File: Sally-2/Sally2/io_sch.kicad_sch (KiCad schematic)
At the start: 41 parts, among them J12 Drive 1-4, J13 OPT, J14 Special_Func, J15 TX GND RX, J16 - RI +, J17 RS232, J18 IN RDY CMD OUT GND, J19 Centronics, U10 MAX232, U11 74LS06, U12 74LS06, U13 Z84C30, U14 74LS244, U15 74LS273, U16 74LS244, U8 74LS273, U9 WD1772_PHY

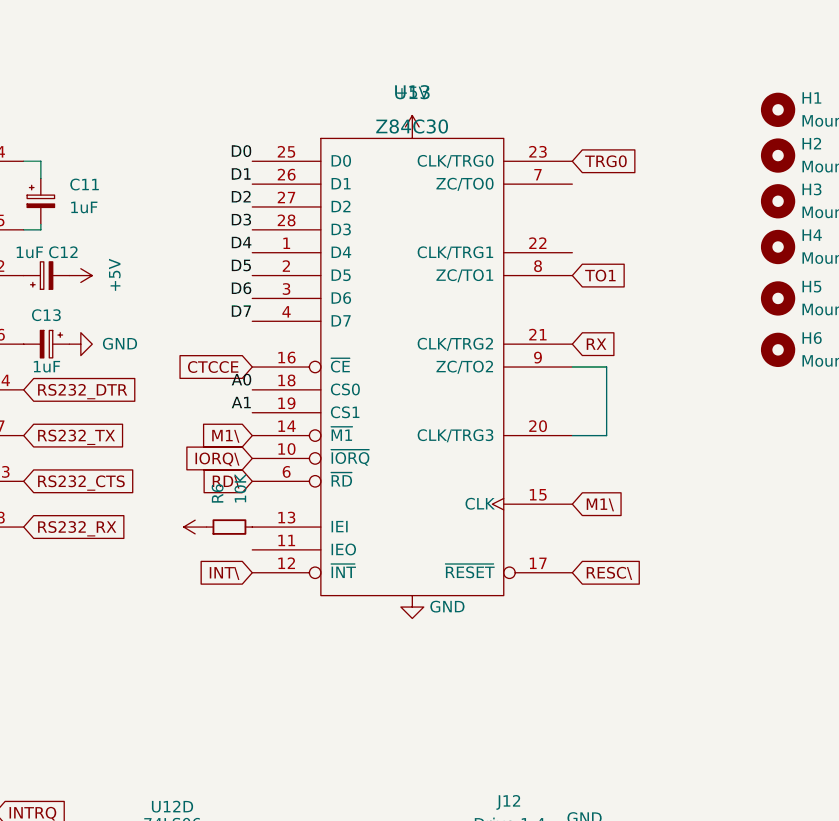
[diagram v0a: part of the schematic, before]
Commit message: Rolli
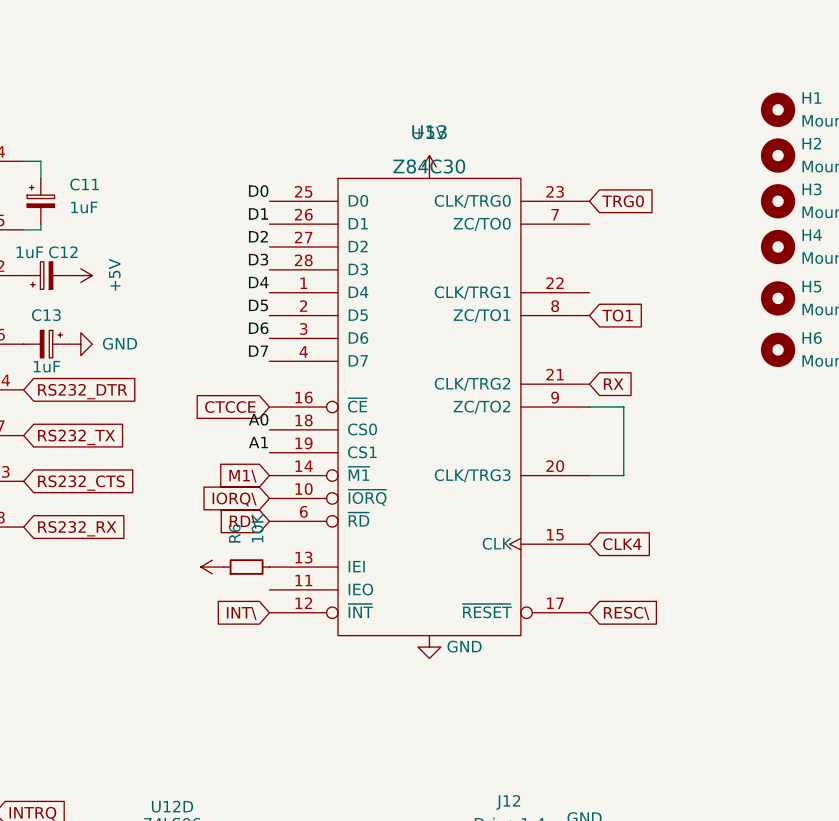
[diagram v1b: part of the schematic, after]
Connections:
- net M1\: no longer U13.15 (CLK)
- new net CLK4: U13.15 (CLK)
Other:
- moved on the sheet: R6, U13
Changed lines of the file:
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@@
 	(wire
 		(pts
-			(xy 132.715 59.055) (xy 128.905 59.055)
+			(xy 134.62 63.5) (xy 130.81 63.5)
 		)
 		(stroke
@@
 	(wire
 		(pts
-			(xy 128.905 51.435) (xy 132.715 51.435)
+			(xy 130.81 55.88) (xy 134.62 55.88)
 		)
 		(stroke
@@
 	(wire
 		(pts
-			(xy 132.715 51.435) (xy 132.715 59.055)
+			(xy 134.62 55.88) (xy 134.62 63.5)
 		)
 		(stroke
@@
 	)
 	(label "A0"
-		(at 93.345 53.975 180)
+		(at 95.25 58.42 180)
 		(fields_autoplaced yes)
 		(effects
@@
 	)
 	(label "D0"
-		(at 93.345 28.575 180)
+		(at 95.25 33.02 180)
 		(fields_autoplaced yes)
 		(effects
@@
 	)
 	(label "D1"
-		(at 93.345 31.115 180)
+		(at 95.25 35.56 180)
 		(fields_autoplaced yes)
 		(effects
@@
 	)
 	(label "D5"
-		(at 93.345 41.275 180)
+		(at 95.25 45.72 180)
 		(fields_autoplaced yes)
 		(effects
@@
 	)
 	(label "D2"
-		(at 93.345 33.655 180)
+		(at 95.25 38.1 180)
 		(fields_autoplaced yes)
 		(effects
@@
 	)
 	(label "D4"
-		(at 93.345 38.735 180)
+		(at 95.25 43.18 180)
 		(fields_autoplaced yes)
 		(effects
@@
 	)
 	(label "D6"
-		(at 93.345 43.815 180)
+		(at 95.25 48.26 180)
 		(fields_autoplaced yes)
 		(effects
@@
 	)
 	(label "D7"
-		(at 93.345 46.355 180)
+		(at 95.25 50.8 180)
 		(fields_autoplaced yes)
 		(effects
@@
 	)
 	(label "D3"
-		(at 93.345 36.195 180)
+		(at 95.25 40.64 180)
 		(fields_autoplaced yes)
 		(effects
@@
 	)
 	(label "A1"
-		(at 93.345 56.515 180)
+		(at 95.25 60.96 180)
 		(fields_autoplaced yes)
 		(effects
@@
 	(global_label "RESC\\"
 		(shape input)
-		(at 128.905 74.295 0)
+		(at 130.81 78.74 0)
 		(fields_autoplaced yes)
 		(effects
@@
 		)
 		(property "Intersheetrefs" "${INTERSHEET_REFS}"
-			(at 137.0633 74.2156 0)
+			(at 138.9683 78.6606 0)
 			(effects
 				(font
@@
 	(global_label "RX"
 		(shape input)
-		(at 128.905 48.895 0)
+		(at 130.81 53.34 0)
 		(fields_autoplaced yes)
 		(effects
@@
 		)
 		(property "Intersheetrefs" "${INTERSHEET_REFS}"
-			(at 133.7976 48.9744 0)
+			(at 135.7026 53.4194 0)
 			(effects
 				(font
@@
 	(global_label "IORQ\\"
 		(shape input)
-		(at 93.345 61.595 180)
+		(at 95.25 66.04 180)
 		(fields_autoplaced yes)
 		(effects
@@
 		)
 		(property "Intersheetrefs" "${INTERSHEET_REFS}"
-			(at 85.5495 61.5156 0)
+			(at 87.4545 65.9606 0)
 			(effects
 				(font
@@
 	(global_label "M1\\"
 		(shape input)
-		(at 93.345 59.055 180)
+		(at 95.25 63.5 180)
 		(fields_autoplaced yes)
 		(effects
@@
 		)
 		(property "Intersheetrefs" "${INTERSHEET_REFS}"
-			(at 87.4243 58.9756 0)
+			(at 89.3293 63.4206 0)
 			(effects
 				(font
@@
 	(global_label "RD\\"
 		(shape input)
-		(at 93.345 64.135 180)
+		(at 95.25 68.58 180)
 		(fields_autoplaced yes)
 		(effects
@@
 		)
 		(property "Intersheetrefs" "${INTERSHEET_REFS}"
-			(at 87.5452 64.0556 0)
+			(at 89.4502 68.5006 0)
 			(effects
 				(font
@@
 	(global_label "TRG0"
 		(shape input)
-		(at 128.905 28.575 0)
+		(at 130.81 33.02 0)
 		(fields_autoplaced yes)
 		(effects
@@
 		)
 		(property "Intersheetrefs" "${INTERSHEET_REFS}"
-			(at 136.0352 28.4956 0)
+			(at 137.9402 32.9406 0)
 			(effects
 				(font
@@
 	(global_label "INT\\"
 		(shape input)
-		(at 93.345 74.295 180)
+		(at 95.25 78.74 180)
 		(fields_autoplaced yes)
 		(effects
@@
 		)
 		(property "Intersheetrefs" "${INTERSHEET_REFS}"
-			(at 87.1824 74.2156 0)
+			(at 89.0874 78.6606 0)
 			(effects
 				(font
@@
 		)
 	)
-	(global_label "M1\\"
-		(shape input)
-		(at 128.905 66.675 0)
-		(fields_autoplaced yes)
-		(effects
-			(font
-				(size 1.27 1.27)
-			)
-			(justify left)
-		)
-		(property "Intersheetrefs" "${INTERSHEET_REFS}"
-			(at 134.8257 66.7544 0)
-			(effects
-				(font
-					(size 1.27 1.27)
-				)
-				(justify left)
-				(hide yes)
-			)
-		)
-	)
 	(global_label "SIORDY"
 		(shape input)
@@
 	(global_label "TO1"
 		(shape input)
-		(at 128.905 41.275 0)
+		(at 130.81 45.72 0)
 		(fields_autoplaced yes)
 		(effects
@@
 		)
 		(property "Intersheetrefs" "${INTERSHEET_REFS}"
-			(at 134.8257 41.1956 0)
+			(at 136.7307 45.6406 0)
 			(effects
 				(font
@@
 	(global_label "CTCCE"
 		(shape input)
-		(at 93.345 51.435 180)
+		(at 95.25 55.88 180)
 		(fields_autoplaced yes)
 		(effects
@@
 		)
 		(property "Intersheetrefs" "${INTERSHEET_REFS}"
-			(at 85.0052 51.3556 0)
+			(at 86.9102 55.8006 0)
 			(effects
 				(font
@@
 		)
 	)
+	(global_label "CLK4"
+		(shape input)
+		(at 130.81 71.12 0)
+		(fields_autoplaced yes)
+		(effects
+			(font
+				(size 1.27 1.27)
+			)
+			(justify left)
+		)
+		(property "Intersheetrefs" "${INTERSHEET_REFS}"
+			(at 138.0007 71.0406 0)
+			(effects
+				(font
+					(size 1.27 1.27)
+				)
+				(justify left)
+				(hide yes)
+			)
+		)
+	)
 	(symbol
 		(lib_id "Mechanical:MountingHole")
@@
 	(symbol
 		(lib_id "Device:R_Small")
-		(at 90.805 69.215 90)
+		(at 92.71 73.66 90)
 		(unit 1)
 		(exclude_from_sim no)
@@
 		(dnp no)
 		(property "Reference" "R6"
-			(at 89.5349 66.675 0)
+			(at 91.4399 71.12 0)
 			(effects
 				(font
@@
 		)
 		(property "Value" "10K"
-			(at 92.0749 66.675 0)
+			(at 93.9799 71.12 0)
 			(effects
 				(font
@@
 		)
 		(property "Footprint" "Resistor_THT:R_Axial_DIN0207_L6.3mm_D2.5mm_P10.16mm_Horizontal"
-			(at 90.805 69.215 0)
+			(at 92.71 73.66 0)
 			(effects
 				(font
@@
 		)
 		(property "Datasheet" "~"
-			(at 90.805 69.215 0)
+			(at 92.71 73.66 0)
 			(effects
 				(font
@@
 		)
 		(property "Description" ""
-			(at 90.805 69.215 0)
+			(at 92.71 73.66 0)
 			(effects
 				(font
@@
 	(symbol
 		(lib_id "power:+5V")
-		(at 111.125 26.035 0)
+		(at 113.03 30.48 0)
 		(unit 1)
 		(exclude_from_sim no)
@@
 		(dnp no)
 		(property "Reference" "#PWR053"
-			(at 111.125 29.845 0)
+			(at 113.03 34.29 0)
 			(effects
 				(font
@@
 		)
 		(property "Value" "+5V"
-			(at 111.125 20.955 0)
+			(at 113.03 25.4 0)
 			(effects
 				(font
@@
 		)
 		(property "Footprint" ""
-			(at 111.125 26.035 0)
+			(at 113.03 30.48 0)
 			(effects
 				(font
@@
 		)
 		(property "Datasheet" ""
-			(at 111.125 26.035 0)
+			(at 113.03 30.48 0)
 			(effects
 				(font
@@
 		)
 		(property "Description" ""
-			(at 111.125 26.035 0)
+			(at 113.03 30.48 0)
 			(effects
 				(font
@@
 	(symbol
 		(lib_id "sergej:Z84C30")
-		(at 111.125 51.435 0)
+		(at 113.03 55.88 0)
 		(unit 1)
 		(exclude_from_sim no)
@@
 		(fields_autoplaced yes)
 		(property "Reference" "U13"
-			(at 111.125 20.955 0)
+			(at 113.03 25.4 0)
 			(effects
 				(font
@@
 		)
 		(property "Value" "Z84C30"
-			(at 111.125 24.765 0)
+			(at 113.03 29.21 0)
 			(effects
 				(font
@@
 		)
 		(property "Footprint" "Package_DIP:DIP-28_W15.24mm"
-			(at 111.125 24.765 0)
+			(at 113.03 29.21 0)
 			(effects
 				(font
@@
 		)
 		(property "Datasheet" ""
-			(at 111.125 59.055 0)
+			(at 113.03 63.5 0)
 			(effects
 				(font
@@
 		)
 		(property "Description" ""
-			(at 111.125 51.435 0)
+			(at 113.03 55.88 0)
 			(effects
 				(font
@@
 	(symbol
 		(lib_id "power:GND")
-		(at 111.125 76.835 0)
+		(at 113.03 81.28 0)
 		(unit 1)
 		(exclude_from_sim no)
@@
 		(fields_autoplaced yes)
 		(property "Reference" "#PWR054"
-			(at 111.125 83.185 0)
+			(at 113.03 87.63 0)
 			(effects
 				(font
@@
 		)
 		(property "Value" "GND"
-			(at 113.03 78.1049 0)
+			(at 114.935 82.5499 0)
 			(effects
 				(font
@@
 		)
 		(property "Footprint" ""
-			(at 111.125 76.835 0)
+			(at 113.03 81.28 0)
 			(effects
 				(font
@@
 		)
 		(property "Datasheet" ""
-			(at 111.125 76.835 0)
+			(at 113.03 81.28 0)
 			(effects
 				(font
@@
 		)
 		(property "Description" ""
-			(at 111.125 76.835 0)
+			(at 113.03 81.28 0)
 			(effects
 				(font
@@
 	(symbol
 		(lib_id "power:+5V")
-		(at 88.265 69.215 90)
+		(at 90.17 73.66 90)
 		(unit 1)
 		(exclude_from_sim no)
@@
 		(dnp no)
 		(property "Reference" "#PWR050"
-			(at 92.075 69.215 0)
+			(at 93.98 73.66 0)
 			(effects
 				(font
@@
 		)
 		(property "Value" "+5V"
-			(at 83.185 72.39 90)
+			(at 85.09 76.835 90)
 			(effects
 				(font
@@
 		)
 		(property "Footprint" ""
-			(at 88.265 69.215 0)
+			(at 90.17 73.66 0)
 			(effects
 				(font
@@
 		)
 		(property "Datasheet" ""
-			(at 88.265 69.215 0)
+			(at 90.17 73.66 0)
 			(effects
 				(font
@@
 		)
 		(property "Description" ""
-			(at 88.265 69.215 0)
+			(at 90.17 73.66 0)
 			(effects
 				(font
